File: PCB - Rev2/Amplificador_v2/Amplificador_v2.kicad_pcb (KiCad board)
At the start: 2 copper layers, 150 x 100 mm, 210 parts, among them IC1 AD817, IC2 AD817, J1 Conn_01x02_Male, J10 Conn_01x02_Male, J11 Screw_Terminal_01x03, J12 Screw_Terminal_01x02, J2 Conn_01x02_Male, J3 Conn_01x02_Male, J4 Conn_01x03_Male, J5 Conn_01x03_Male, J6 Screw_Terminal_01x02, J7 Conn_01x02_Male, J8 Conn_01x03_Male, J9 Screw_Terminal_01x03, Q1 BC847, Q10 BC847, Q11 BC857, Q12 BC847, Q13 2N7002, Q14 BC847, Q15 BC857, Q16 PHB27NQ10T, Q17 PHB27NQ10T, Q2 BC847, Q3 BC847, Q4 2N7002, Q5 BC857, Q6 BC847, Q7 BC847, Q8 BC857, Q9 BC857, U1 TL082, U10 LM7805_TO220, U11 NE5532, U12 NE5532, U2 LM311, U3 LM311, U4 SN74LVC2G02DCUR, U5 LM311, U6 UCC20520DWR, U7 LM7812_TO220, U8 LM7815_TO220, U9 LM7915_TO220

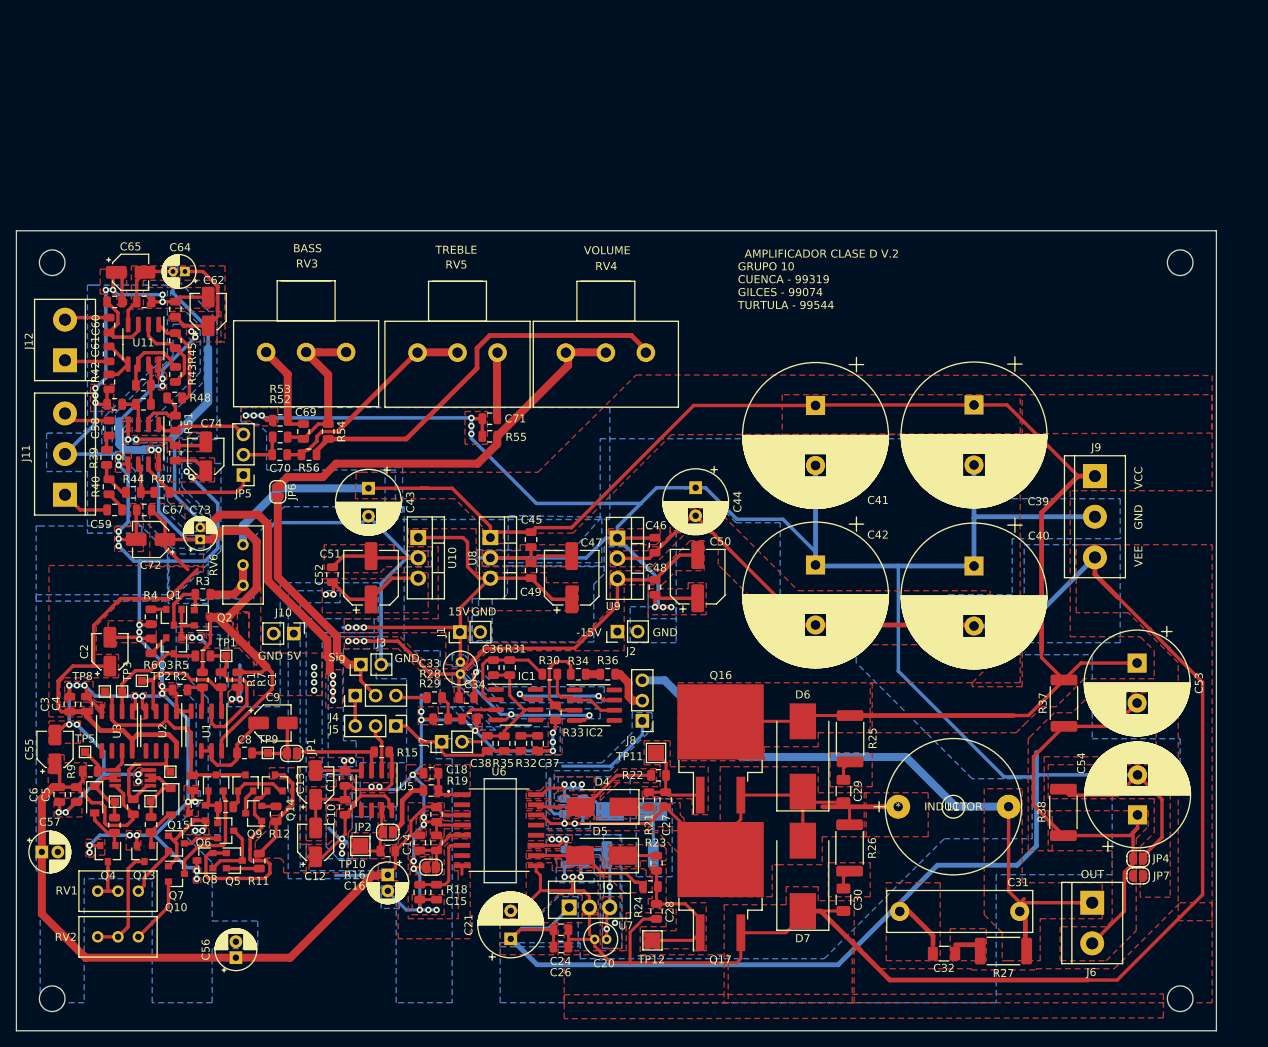
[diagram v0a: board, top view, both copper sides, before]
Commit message: Terminado esto
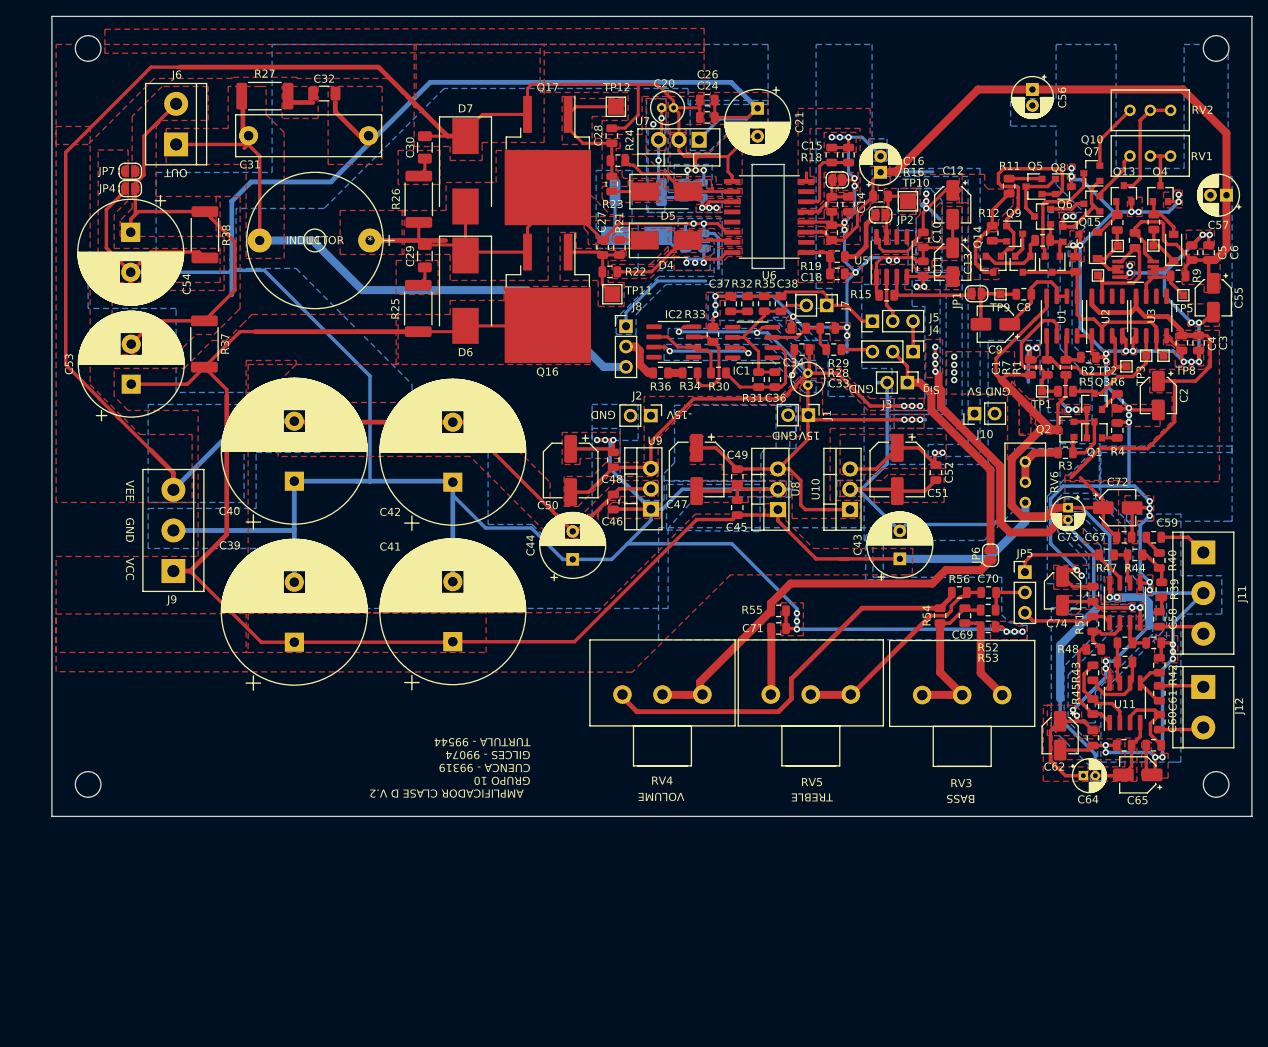
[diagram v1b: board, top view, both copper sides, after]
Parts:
- moved REF** 187.8 mm to (195.5, 56.7), turned to 180 degrees
- moved REF** 181.0 mm to (54.5, 56.7), turned to 180 degrees
- moved C57 169.3 mm to (196.8, 75.1), turned to 180 degrees
- moved RV2 161.4 mm to (184.7, 64.5), turned to 180 degrees
- moved REF** 159.4 mm to (195.5, 148.7), turned to 180 degrees
- moved C6 158.8 mm to (194.6, 82.2), turned to 90 degrees
- moved C55 155.4 mm to (195.1, 87.9), turned to 270 degrees
- moved Q4 155.3 mm to (188.5, 74.9), turned to 90 degrees
- moved C5 155.0 mm to (192.5, 82.2), turned to 90 degrees
- moved RV1 154.3 mm to (184.7, 70.2), turned to 180 degrees
- moved JP7 153.7 mm to (59.8, 72.1), turned to 0 degrees
- moved D1 151.5 mm to (190.2, 81.6), turned to 90 degrees
- moved REF** 151.3 mm to (54.5, 148.7), turned to 180 degrees
- moved JP4 151.3 mm to (59.8, 74.2), turned to 0 degrees
- moved R10 150.2 mm to (187.7, 78.4), turned to 270 degrees
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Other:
- outline, holes or cut-outs redrawn
